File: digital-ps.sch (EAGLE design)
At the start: 83 parts, among them CON1 SWD_CON, IC1 STM32F334K8, IC2 MCP14700, IC3 7805, IC4 7805, IC5 3.3V, Q1 40V, Q2 40V, X1 12MHz

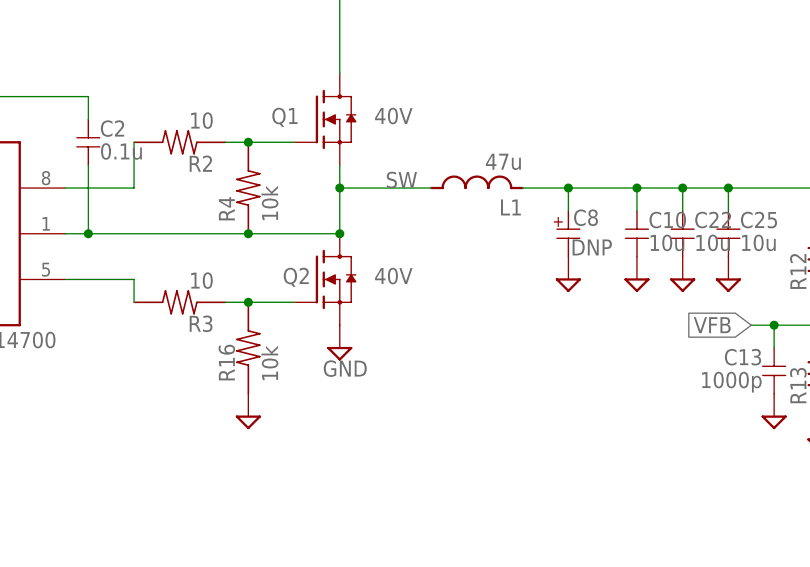
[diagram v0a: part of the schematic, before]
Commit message: 微修正
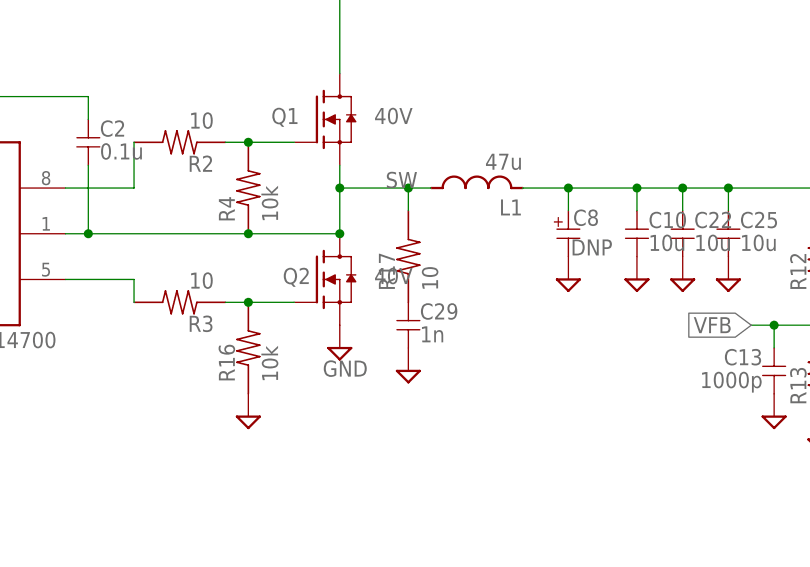
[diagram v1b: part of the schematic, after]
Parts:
- added C29: 1n, my_rcl:C-1608
- added R17: 10, my_rcl:R-2012
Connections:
- new net N$28: C29.1, R17.1
- net GND: now also C29.2
- net SW: now also R17.2

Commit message: 微修正
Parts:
- removed TP12: PA12, my_connector:TESTPIN
- removed TP13: PA11, my_connector:TESTPIN
- removed TP14: PA10, my_connector:TESTPIN
- added C30, C31, C33, C34: 10u, my_rcl:C-3225-2
- added C32: DNP, my_rcl:CPOLE5-13
- added C35, C36, C37, C39, C40: 1u, my_rcl:C-1608-2
- added C38: 0.1u, my_rcl:C-1608-2
- added C41: 1u, my_rcl:C-2012-2
- added D2, D3: SBD-1A2, my_rcl:SBD-1A2
- added FB2: FB, my_rcl:FB
- added FB3, FB4: FB, my_rcl:FB-1608FB
- added R18: 10m, my_rcl:R-6432
- added R19: 2, my_rcl:R-1608-2
- added T1: COMMON_FILTER-SMALL, my_rcl:COMMON_FILTER-SMALL
- added TP24: +3V3, my_connector:TESTPIN
- added TP25, TP27: GND, my_connector:TESTPIN
- added TP26: +5V, my_connector:TESTPIN
- C1: device my_rcl:C-2012 -> my_rcl:C-3216
- C10, C9: value 10u -> 10p; device my_rcl:C-3216 -> my_rcl:C-1608
- C11: value 10u -> 1000p; device my_rcl:C-3216 -> my_rcl:C-1608
- C12: value 0.1u -> 1000p
- C15: value 1000p -> 10u; device my_rcl:C-1608 -> my_rcl:C-2012
- C16: value 1000p -> 0.1u
- C18: value DNP -> 1000p; device my_rcl:CPOLE5-13 -> my_rcl:C-1608
- C20: value 10u -> 1000u; device my_rcl:C-3216 -> my_rcl:CPOLE5-13
- C22, C23: device my_rcl:C-3216 -> my_rcl:C-3225-2
- C24: value 10u -> 1u; device my_rcl:C-3216 -> my_rcl:C-1608-2
- C25: value 10u -> 1n; device my_rcl:C-3216 -> my_rcl:C-1608-2
- C26: value 10p -> DNP; device my_rcl:C-1608 -> my_rcl:CPOLE5-13
- C27: value 10p -> 1u; device my_rcl:C-1608 -> my_rcl:C-1608-2
- C28: value 0.1u -> 10u; device my_rcl:C-1608 -> my_rcl:C-3225-2
- C29: value 1n -> 10u; device my_rcl:C-1608 -> my_rcl:C-3225-2
- C5: value 1000u -> 10u; device my_rcl:CPOLE5-13 -> my_rcl:C-2012
- C6: value 1u -> 0.1u; device my_rcl:C-2012 -> my_rcl:C-1608
- C7: value 10u -> 0.1u; device my_rcl:C-3216 -> my_rcl:C-1608
- C8: value DNP -> 0.1u; device my_rcl:CPOLE5-13 -> my_rcl:C-1608
- IC1: value STM32F334K8 -> 7805; device my_ic:STM32F334K8 -> my_ic:78X-3
- IC2: value MCP14700 -> 3.3V; device my_ic:MCP14700 -> my_ic:78X-SOP
- IC3: value 7805 -> STM32F334K8; device my_ic:78X-SOP -> my_ic:STM32F334K8
- IC4: value 7805 -> OPA; device my_ic:78X-SOP -> my_ic:OPA-2-SOP
- IC5: value 3.3V -> MCP14700; device my_ic:78X-SOP -> my_ic:MCP14700
- Q1, Q2: value 40V -> EPC2052
- R1: value 1M -> 120; device my_rcl:R-2012 -> my_rcl:R-1608
- R10: value 10k -> 100
- R11, R12: value 10k -> 10; device my_rcl:R-1608 -> my_rcl:R-2012
- R13: value 1k -> 10k; device my_rcl:R-1608 -> my_rcl:R-2012
- R14: value 100 -> 10k; device my_rcl:R-1608 -> my_rcl:R-2012
- R15: value 100 -> 10; device my_rcl:R-1608 -> my_rcl:R-1608-2
- R16, R4: device my_rcl:R-2012 -> my_rcl:R-1608
- R17: value 10 -> 1k; device my_rcl:R-2012 -> my_rcl:R-1608
- R2: value 10 -> 120; device my_rcl:R-2012 -> my_rcl:R-1608
- R3: value 10 -> 10k; device my_rcl:R-2012 -> my_rcl:R-1608
- R5: value 120 -> 10k
- R6: value 120 -> 1k
- R7: value 40m -> 1k; device my_rcl:R-6432 -> my_rcl:R-1608
- R8: value 1k -> 1M
- R9: value 1k -> 100
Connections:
- removed net N$20: IC1.PA10, TP14.1
- removed net N$21: IC1.PA11, TP13.1
- removed net N$22: IC1.PA12, TP12.1
- removed net VCC: C20.1, FB1.2, IC3.IN, IC4.IN
- new net IN+: C41.1, T1.4, TP5.1
- new net IN-: C41.2, T1.1, TP6.1
- new net N$29: C11.1, IC4G$2.-IN, R3.2, R6.1
- new net N$30: C12.1, IC3.PA6, IC4G$1.OUT, R4.1
- new net N$31: C14.1, IC3.PA5, IC4G$1.+IN
- new net N$32: FB3.1, R11.1, R13.2
- new net N$33: FB4.1, R12.1, R14.2
- new net N$34: C38.1, R19.1
- net +3V3: now also C19.1, C6.1, C7.1, C8.1, IC2.OUT, IC3.VDDA/VREF+, IC3.VDD_1, IC3.VDD_2, IC4G$3.V+, R8.2, TP24.1; no longer C12.1, C21.1, C28.1, IC1.VDDA/VREF+, IC1.VDD_1, IC1.VDD_2, IC5.OUT, R1.1
- net +5V: now also C5.1, FB2.1, IC1.OUT, IC2.IN, TP26.1; no longer IC4.OUT, IC5.IN
- net +5VP: now also C15.1, C16.1, FB2.2, IC5.VCC; no longer C1.1, C19.1, IC2.VCC, IC3.OUT
- net GND: now also C10.1, C15.2, C17.1, C18.2, C2.2, C23.2, C24.2, C26.2, C27.2, C30.2, C35.2, C36.2, C37.2, C38.2, C39.2, C9.1, D3.A, IC1.GND, IC3.BOOT0, IC3.VSS_1, IC3.VSS_2, IC4G$3.V-, R14.1, R17.1, R18.1, R5.1, R9.2, T1.2, TP25.1, TP27.1; no longer C10.2, C12.2, C15.1, C21.2, C26.1, C27.1, C9.2, IC1.BOOT0, IC1.VSS_1, IC1.VSS_2, IC3.GND, IC4.GND, R11.1, R13.1, R14.2, R16.1, R7.1, TP6.1
- net N$1: now also IC3.PA8, R2.1; no longer IC1.PA8, R6.1
- net N$10: now also FB4.2; no longer R16.2, R3.1
- net N$11: now also C18.1, R10.1, R7.2; no longer C14.1, R15.1, R9.2
- net N$12: now also IC5.LOWDR, R12.2; no longer IC2.LOWDR, R3.2
- net N$13: now also IC3.PA3; no longer IC1.PA3
- net N$14: now also IC3.PA4; no longer IC1.PA4
- net N$15: now also IC3.PA0; no longer IC1.PA0
- net N$16: now also IC3.PA1; no longer IC1.PA1
- net N$17: now also IC3.PA2; no longer IC1.PA2
- net N$18: now also IC3.PB7; no longer IC1.PB7
- net N$19: now also IC3.PB5; no longer IC1.PB5
- net N$2: now also IC3.PA9, R1.1; no longer IC1.PA9, R5.1
- net N$23: now also IC3.PB4; no longer IC1.PB4
- net N$24: now also C10.2, IC3.PF0/OSC_IN; no longer C26.2, IC1.PF0/OSC_IN
- net N$25: now also C9.2, IC3.PF1_OSC_OUT; no longer C27.2, IC1.PF1_OSC_OUT
- net N$26: now also IC3.PB3; no longer IC1.PB3
- net N$27: now also IC3.PA15; no longer IC1.PA15
- net N$28: now also C25.1, R15.1; no longer C29.1, R17.1
- net N$3: now also C11.2, IC3.PB0, IC4G$2.OUT, R3.1; no longer C17.2, IC1.PA6, R10.1
- net N$4: now also C1.1, C2.1, FB1.2, IC1.IN; no longer C17.1, IC1.PA5, R10.2, R8.1
- net N$5: now also C13.1, IC4G$2.+IN, R5.2, R7.1, R8.1; no longer C16.1, IC1.PA7, R1.2, R11.2, R9.1
- net N$6: now also IC5.HIGHDR, R11.2; no longer IC2.HIGHDR, R2.2
- net N$7: now also C21.1, IC5.BOOT; no longer C2.1, IC2.BOOT
- net N$8: now also C17.2, R6.2, R9.1; no longer C15.2, R14.1, R8.2
- net N$9: now also FB3.2; no longer R2.1, R4.2
- net OUT+: now also C26.1, C27.1, C28.1, C29.1, C30.1, C31.1, C32.1, C33.1, C34.1, C39.1, C40.1, R16.2; no longer C10.1, C11.1, C18.1, C22.1, C23.1, C24.1, C25.1, C8.1, R12.2
- net OUT-: now also C31.2, C32.2, C33.2, C34.2, C40.2, R10.2, R18.2; no longer C11.2, C18.2, C23.2, C24.2, R15.2, R7.2
- net PWMH: now also IC5.HI, R1.2; no longer IC2.HI, R5.2
- net PWML: now also IC5.LI, R2.2; no longer IC2.LI, R6.2
- net SW: now also C21.2, D2.A, D3.K, IC5.PHASE, R13.1, R15.2; no longer C2.2, IC2.PHASE, R17.2, R4.1
- net SWCLK: now also IC3.SWCLK; no longer IC1.SWCLK
- net SWDIO: now also IC3.SWDIO; no longer IC1.SWDIO
- net UART_TX: now also IC3.PB6; no longer IC1.PB6
- net VFB: now also C12.2, IC4G$1.-IN, R16.1, R17.2, R4.2; no longer C13.1, IC1.PB0, IC1.PB1, R12.1, R13.2
- net VP: now also C20.1, C22.1, C23.1, C24.1, C35.1, C36.1, C37.1, D2.K, R19.2, T1.3; no longer C5.1, C6.1, C7.1, C9.1, TP5.1
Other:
- moved on the sheet: C1, C10, C11, C12, C13, C14, C15, C16, C17, C19, C2, C21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

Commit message: Si
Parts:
- removed FB3, FB4: FB, my_rcl:FB-1608FB
- removed R19: 2, my_rcl:R-1608-2
- added T2: COMMON_FILTER-SMALL, my_rcl:COMMON_FILTER-SMALL
- C1: value 10u -> 1u; device my_rcl:C-3216 -> my_rcl:C-2012-2
- C11: value 1000p -> 10p
- C15: value 10u -> 1000p; device my_rcl:C-2012 -> my_rcl:C-1608
- C16, C7: value 0.1u -> 10u; device my_rcl:C-1608 -> my_rcl:C-2012
- C17: value 1000p -> 0.1u
- C18: value 1000p -> 1u; device my_rcl:C-1608 -> my_rcl:C-1608-2
- C19: value 0.1u -> 1u; device my_rcl:C-1608 -> my_rcl:C-1608-2
- C2: value 0.1u -> 10u; device my_rcl:C-1608 -> my_rcl:C-3216
- C20: value 1000u -> 1000p; device my_rcl:CPOLE5-13 -> my_rcl:C-1608
- C21: value 0.1u -> 1000p
- C22, C33, C34: value 10u -> 1u; device my_rcl:C-3225-2 -> my_rcl:C-1608-2
- C23: value 10u -> 0.1u; device my_rcl:C-3225-2 -> my_rcl:C-1608
- C24: value 1u -> 1000u; device my_rcl:C-1608-2 -> my_rcl:CPOLE5-13
- C25: value 1n -> 10u; device my_rcl:C-1608-2 -> my_rcl:C-3225-2
- C26: value DNP -> 10u; device my_rcl:CPOLE5-13 -> my_rcl:C-3225-2
- C27: value 1u -> 0.1u; device my_rcl:C-1608-2 -> my_rcl:C-1608
- C3: value 10u -> 0.1u; device my_rcl:C-2012 -> my_rcl:C-1608
- C30: value 10u -> 1u
- C31: value 10u -> 0.1u
- C35, C36, C37, C39, C40: value 1u -> 10u; device my_rcl:C-1608-2 -> my_rcl:C-3225-2
- C38: value 0.1u -> 470u; device my_rcl:C-1608-2 -> my_rcl:CPOLE5-13
- C41: device my_rcl:C-2012-2 -> my_rcl:C-1608-2
- C9: value 10p -> 0.1u
- FB1: value FB-2012 -> FB-1608FB; device my_rcl:FB-2012 -> my_rcl:FB-1608FB
- IC1: value 7805 -> 3.3V; device my_ic:78X-3 -> my_ic:78X-SOP
- IC2: value 3.3V -> 7805; device my_ic:78X-SOP -> my_ic:78X-3
- Q1, Q2: device my_ic:NMOSEPC2052 -> my_ic:NMOS-DFN
- R10, R9: value 100 -> 39
- R15: value 10 -> 10k; device my_rcl:R-1608-2 -> my_rcl:R-1608
- R16: value 10k -> 1k
- R17: value 1k -> 10m; device my_rcl:R-1608 -> my_rcl:R-6432
- R18: value 10m -> DNP; device my_rcl:R-6432 -> my_rcl:R-1608
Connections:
- removed net N$10: FB4.2, Q2.G
- removed net N$28: C25.1, R15.1
- removed net N$34: C38.1, R19.1
- removed net N$9: FB3.2, Q1.G
- new net ISENSE: R10.2, R17.2, T2.1
- new net OUT: C32.1, C33.1, C34.1, C35.1, C36.1, L1.2, R15.2, T2.4
- net +3V3: now also C23.1, C9.1, IC1.OUT; no longer C19.1, C7.1, IC2.OUT
- net +5V: now also C7.1, IC1.IN, IC2.OUT; no longer C3.1, IC1.OUT, IC2.IN
- net +5VP: now also C17.1; no longer C15.1
- net GND: now also C11.1, C17.2, C20.1, C21.2, C31.2, C32.2, C33.2, C34.2, C9.2, R16.1; no longer C1.2, C13.2, C17.1, C20.2, C27.2, C37.2, C38.2, C39.2, C9.1, R18.1
- net IN+: now also C1.1; no longer C41.1
- net IN-: now also C1.2; no longer C41.2
- net N$11: now also C21.1; no longer C18.1
- net N$24: now also C11.2; no longer C10.2
- net N$25: now also C10.2; no longer C9.2
- net N$29: now also C12.1; no longer C11.1
- net N$3: now also C12.2; no longer C11.2
- net N$30: now also C13.1; no longer C12.1
- net N$31: now also C15.1; no longer C14.1
- net N$32: now also Q1.G; no longer FB3.1
- net N$33: now also Q2.G; no longer FB4.1
- net N$4: now also C3.1, IC2.IN; no longer C1.1, IC1.IN
- net N$5: now also C14.1; no longer C13.1
- net N$7: now also C27.1; no longer C21.1
- net N$8: now also C20.2; no longer C17.2
- net OUT+: now also C37.1, C38.1, C41.1, R18.2, T2.3; no longer C26.1, C27.1, C28.1, C29.1, C30.1, C31.1, C32.1, C33.1, C34.1, L1.2, R16.2
- net OUT-: now also C37.2, C38.2, C39.2, C41.2, T2.2; no longer C31.2, C32.2, C33.2, C34.2, R10.2, R18.2
- net SW: now also C27.2; no longer C21.2, R15.2
- net VFB: now also C13.2, R15.1, R16.2, R18.1; no longer C12.2, R16.1, R17.2
- net VP: now also C18.1, C19.1, C25.1, C26.1, C28.1, C29.1, C30.1, C31.1; no longer C20.1, C23.1, C35.1, C36.1, C37.1, R19.2
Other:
- moved on the sheet: C1, C10, C11, C12, C13, C14, C15, C16, C17, C18, C19, C2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
